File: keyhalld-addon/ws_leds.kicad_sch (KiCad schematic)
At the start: 9 parts

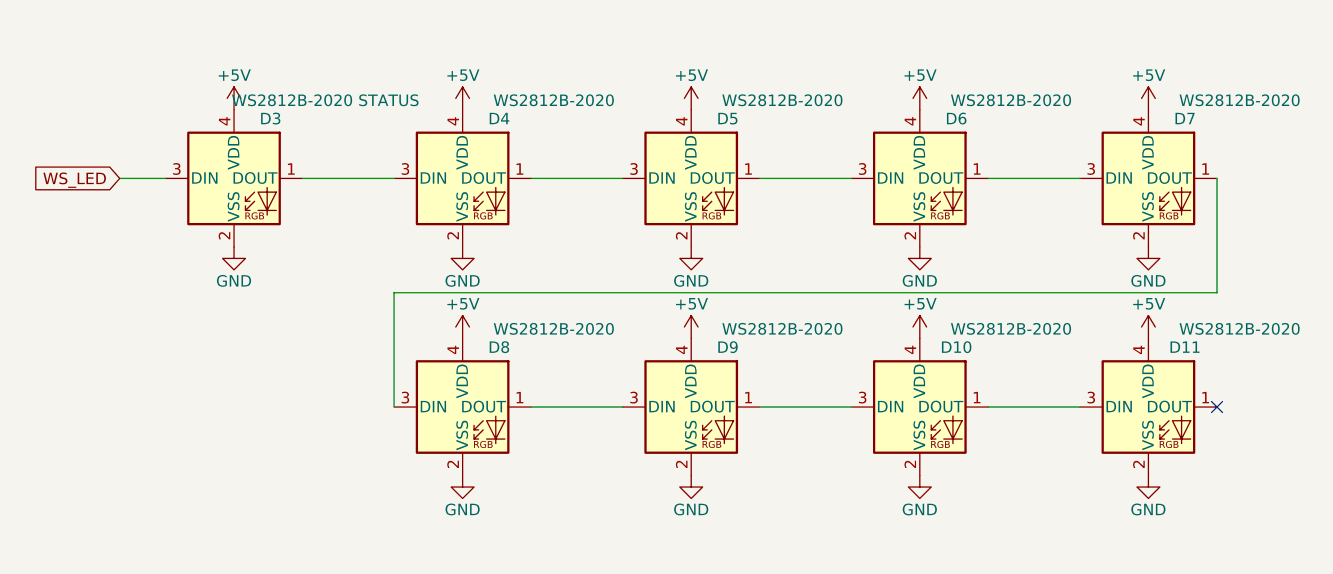
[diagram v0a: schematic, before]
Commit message: routed pcb for addon board
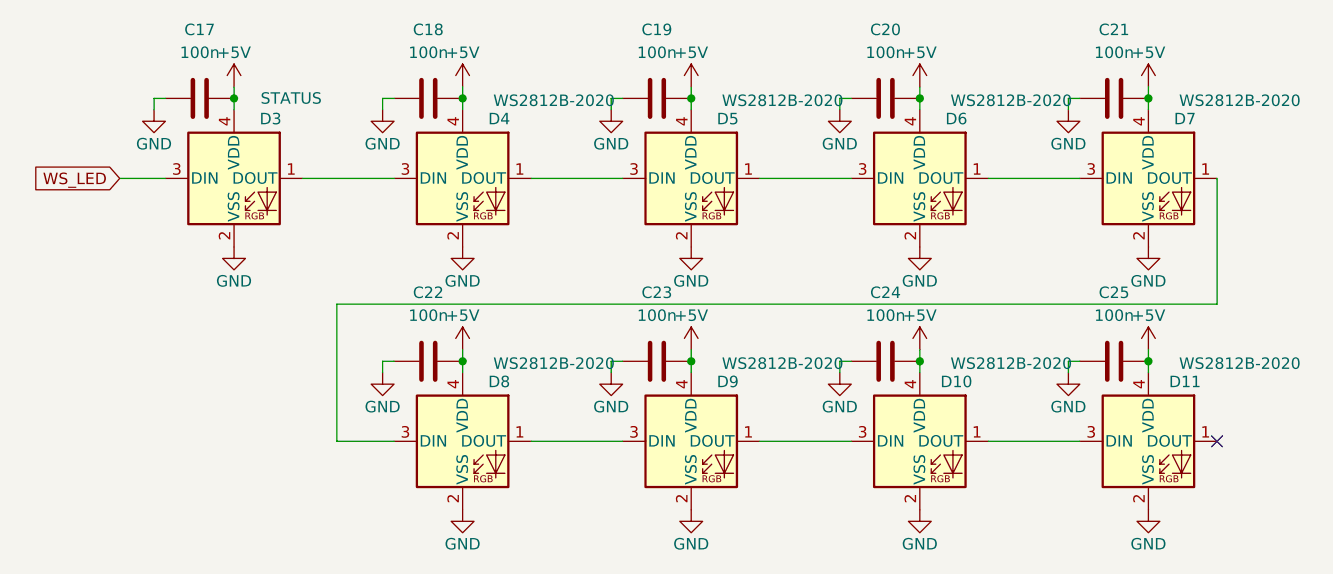
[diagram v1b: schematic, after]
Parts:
- added C17, C18, C19, C20, C21, C22, C23, C24, C25: 100n, Capacitor_SMD:C_0603_1608Metric, symbol Device:C
- D3: value WS2812B-2020 STATUS -> STATUS
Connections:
- net +5V: now also C17.2, C18.2, C19.2, C20.2, C21.2, C22.2, C23.2, C24.2, C25.2
- net GND: now also C17.1, C18.1, C19.1, C20.1, C21.1, C22.1, C23.1, C24.1, C25.1
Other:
- moved on the sheet: D10, D11, D8, D9
